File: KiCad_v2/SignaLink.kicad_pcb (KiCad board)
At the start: 2 copper layers, 59.7 x 45 mm, 72 parts, among them U1 MT3608, U2 ESP32-C3_SUPERMINI_TH, U3 DM-OLED096-636, U4 MPU-6050, U5 BNO085, U6 MCP73871, U7 LTC4415IMSE_PBF, U8 TPS54331

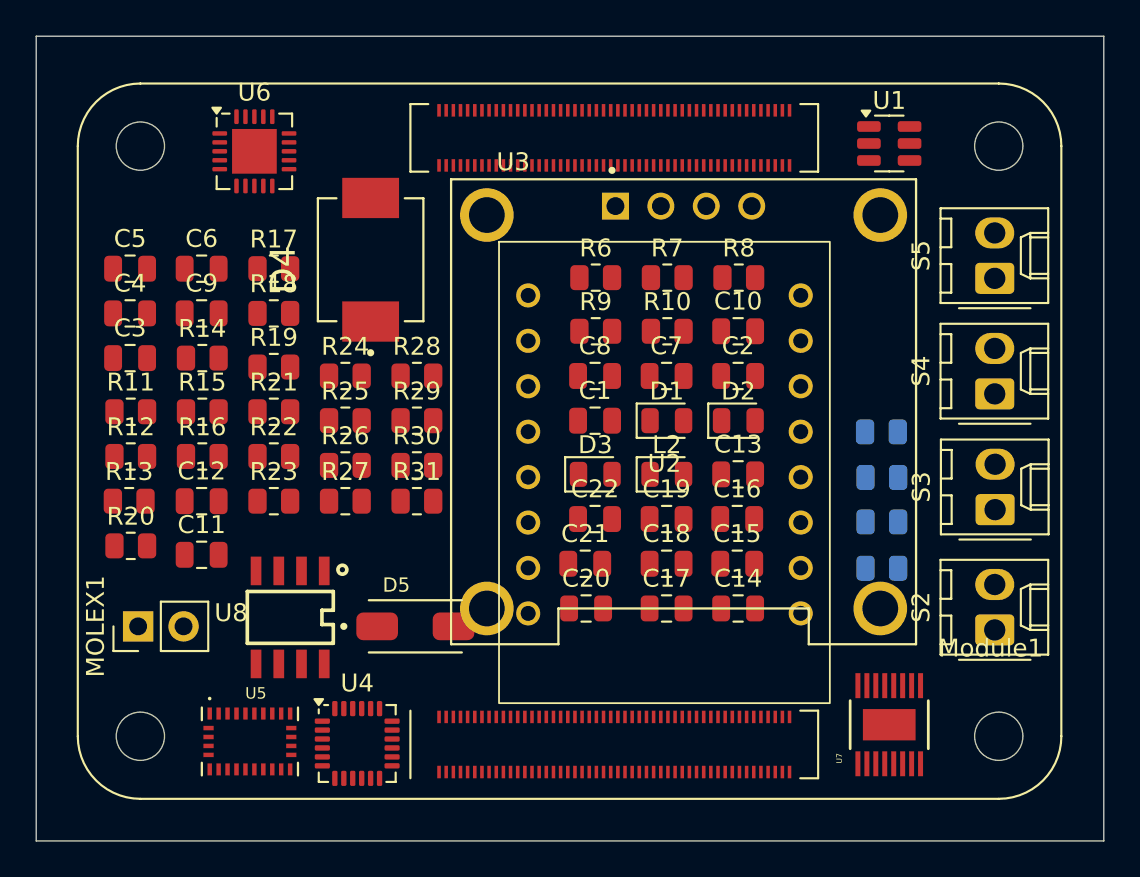
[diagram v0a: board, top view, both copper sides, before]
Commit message: chore: pocos cambios
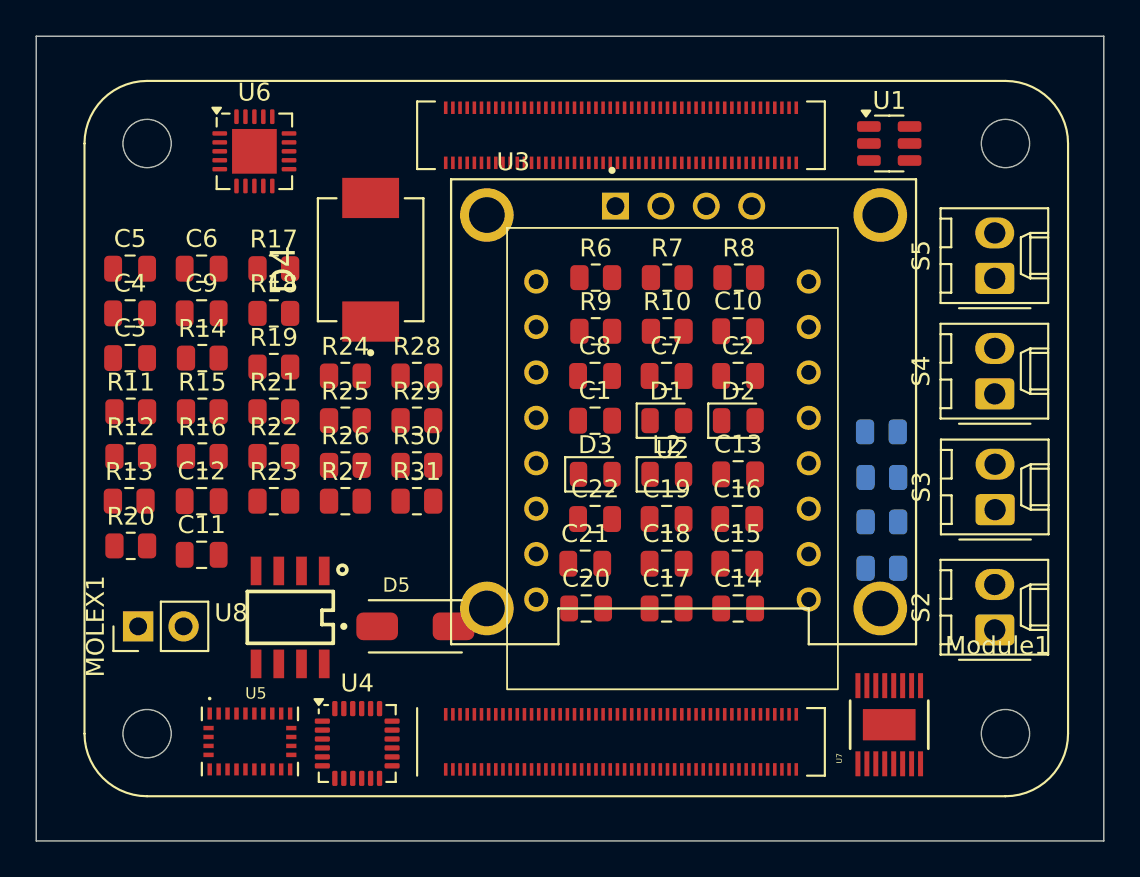
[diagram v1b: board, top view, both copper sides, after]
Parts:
- moved U2 0.90 mm to (69.4, 70.6)
- moved Module1 0.40 mm to (88.0, 86.0)
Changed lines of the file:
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@@
 	(footprint "CM4IO:Raspberry-Pi-4-Compute-Module"
 		(layer "F.Cu")
-		(at 87.625 86.145 90)
+		(at 88 86 90)
 		(descr "Raspberry Pi 4 Compute Module")
 		(tags "Raspberry Pi 4 Compute Module")
@@
 		)
 		(embedded_fonts no)
-		(model "${KICAD_3DMODELS}/CM4.step"
+		(model "${KIPRJMOD}/libs/3dmodels/CM4.step"
 			(offset
-				(xyz 52.4 51.5 -2.8)
+				(xyz -19.3 -3 -2.8)
 			)
 			(scale
@@
 			)
 			(rotate
-				(xyz -0 -180 -90)
+				(xyz -180 -0 -90)
 			)
 		)
@@
 	(footprint "Custom_Footprints:MODULE_ESP32-C3_SUPERMINI_TH"
 		(layer "F.Cu")
-		(at 68.93 71.395)
+		(at 69.38 70.62)
 		(property "Reference" "U2"
 			(at 0 -0.5 0)
@@
 		)
 		(embedded_fonts no)
-		(model "${KICAD_3DMODELS}/ESP32-C3_SUPERMINI_TH.step"
+		(model "${KIPRJMOD}/libs/3dmodels/ESP32-C3_SUPERMINI_TH.step"
 			(offset
 				(xyz 0 0 0)
